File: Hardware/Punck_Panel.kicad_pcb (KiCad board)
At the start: 2 copper layers, 91.2 x 128.5 mm, 40 parts

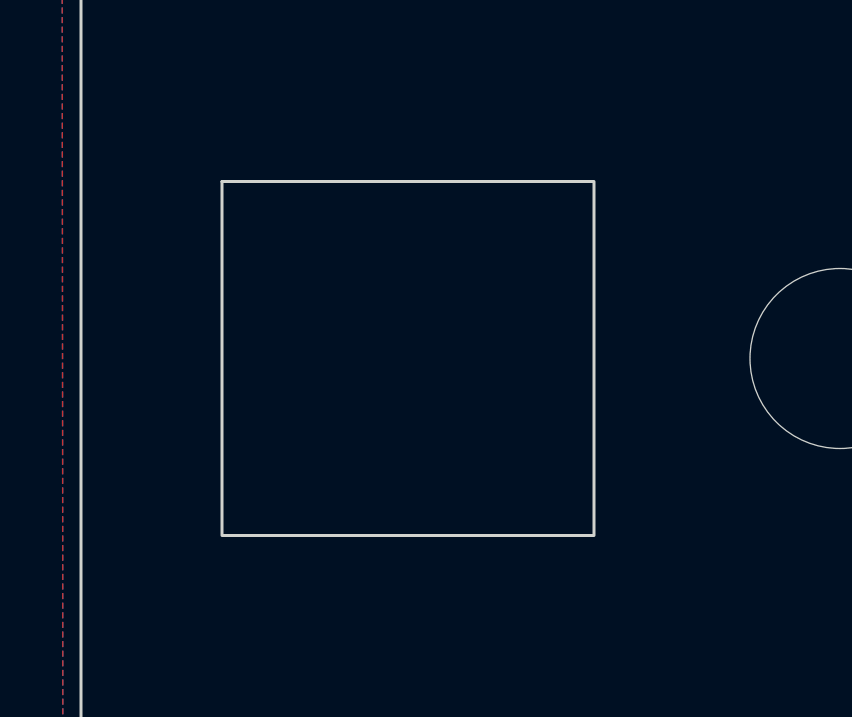
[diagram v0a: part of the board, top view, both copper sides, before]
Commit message: More PCB tweaking
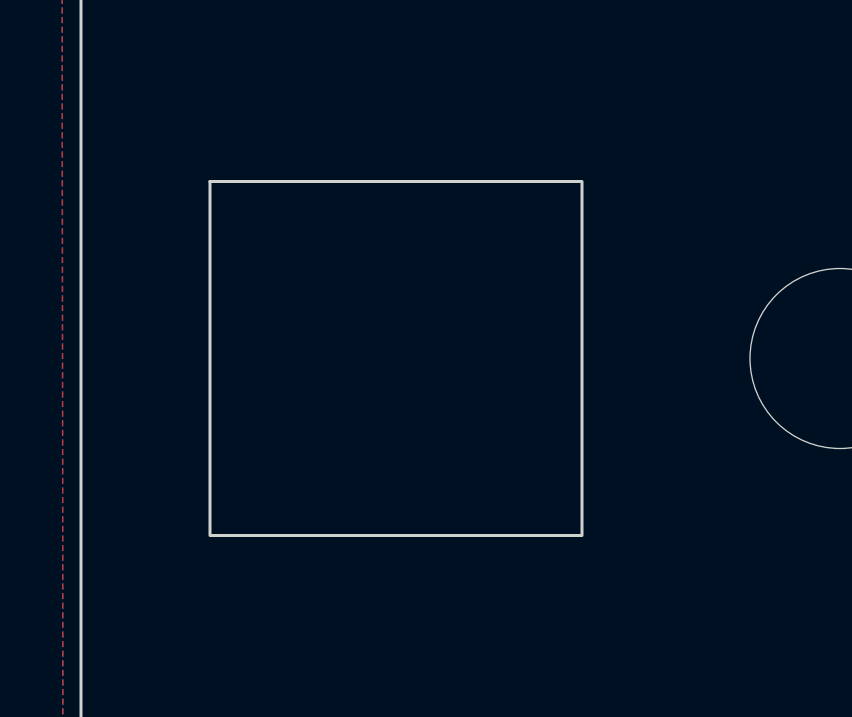
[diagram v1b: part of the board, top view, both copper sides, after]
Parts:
- moved USB** 0.40 mm to (80.4, 150.0)
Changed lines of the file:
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@@
   )
   (footprint "Custom_Footprints:USB_B_CUTOUT" (layer "F.Cu")
-    (at 80.8 150)
+    (at 80.4 150)
     (attr smd)
     (fp_text reference "USB**" (at 0 -7 unlocked) (layer "F.SilkS") hide
